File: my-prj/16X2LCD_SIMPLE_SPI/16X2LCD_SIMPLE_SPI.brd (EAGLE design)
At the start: 75.9 x 33 mm, 10 parts, among them IC1 4094D, U1 LCD-16X2SILK

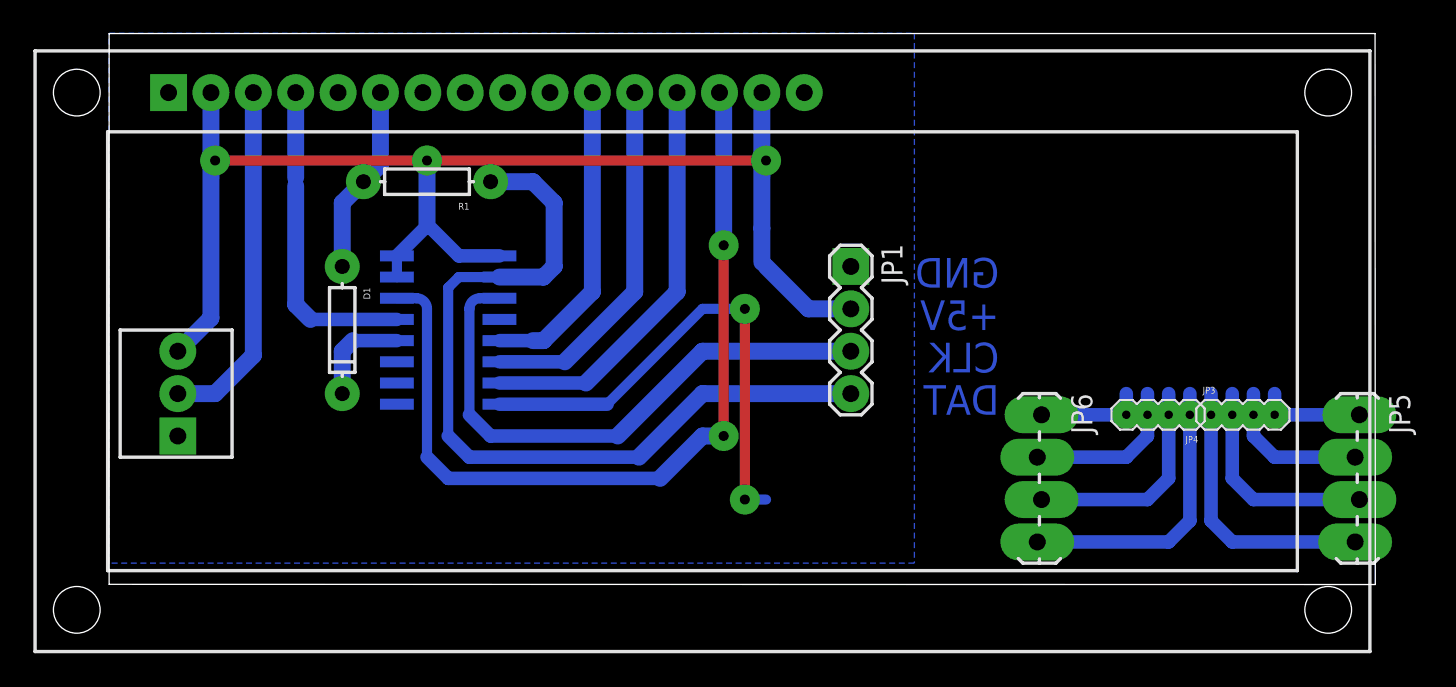
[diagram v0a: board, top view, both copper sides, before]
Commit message: t
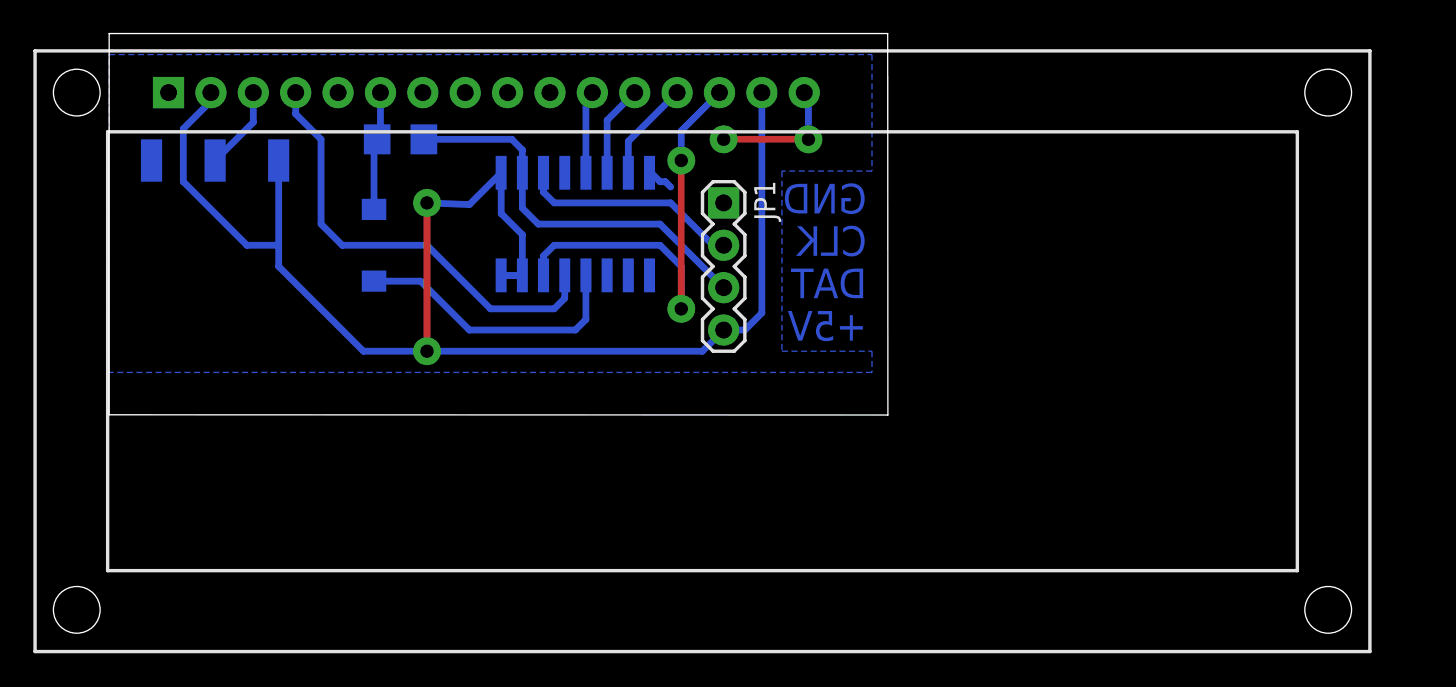
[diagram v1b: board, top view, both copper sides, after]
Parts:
- removed JP3, JP4: (no value), SparkFun-Connectors:1X04-1.27MM
- removed JP5, JP6: (no value), SparkFun:1X04_LOCK_LONGPADS
- removed R3: TRIMPOT, SparkFun:3362U-2
- added U$1: TRIMPOT_S3_SMD, custom:TRIMPOT_S3_SMD
- D1: device SparkFun:DIODE-1N4148 -> SparkFun-DiscreteSemi:SMA-DIODE
- R1: device SparkFun:AXIAL-0.3 -> SparkFun-Passives:1206
- moved IC1 9.92 mm to (39.4, 25.4), turned to 180 degrees
- moved JP1 8.52 mm to (48.3, 26.7)
- moved D1 5.43 mm to (27.3, 24.1), flipped to the bottom
- moved R1 3.00 mm to (28.9, 30.5), flipped to the bottom, turned to 0 degrees
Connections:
- removed net N$11: JP3.3, JP5.2
- removed net N$12: JP3.4, JP5.1
- removed net N$13: JP4.1, JP6.4
- removed net N$14: JP4.2, JP6.3
- removed net N$15: JP4.3, JP6.2
- removed net N$16: JP4.4, JP6.1
- removed net N$5: JP3.1, JP5.4
- removed net N$8: JP3.2, JP5.3
- net CLK: now also JP1.2; no longer JP1.3
- net DATA: now also JP1.3, R1.1; no longer JP1.4, R1.P$1
- net GND: now also U$1.P$1; no longer R3.1
- net N$2: now also R1.2; no longer R1.P$2
- net N$3: now also U$1.P$2; no longer R3.2
- net VDD: now also JP1.4, U$1.P$3; no longer JP1.2, R3.3
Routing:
- net DATA: track 50.1 -> 23.7 mm
- net N$10: track 51.1 -> 26.7 mm
- net CLK: track 33.9 -> 13.3 mm
- net GND: track 29.8 -> 9.61 mm
- net N$9: track 24.9 -> 6.02 mm
- net N$13: track 17.3 -> 0.00 mm
- net N$5: track 16.8 -> 0.00 mm
- net N$7: track 21.8 -> 5.49 mm
- net N$3: track 21.2 -> 5.02 mm
- net N$6: track 18.7 -> 4.97 mm
- net N$8: track 13.2 -> 0.00 mm
- net N$14: track 13.2 -> 0.00 mm
- net N$4: track 6.08 -> 16.8 mm
- net N$15: track 9.67 -> 0.00 mm
- net N$11: track 9.16 -> 0.00 mm
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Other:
- board size 75.9 x 33 mm -> 46.7 x 22.9 mm
